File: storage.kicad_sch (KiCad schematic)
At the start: 26 parts, among them J4 uSD card, J5 uSD card, P1 uBUS2, P2 uBUS1, Q1 BC856, Q2 BC856, U10 IS61WV20488BLL-10TLI, U11 MT48LC16M16A2TG, U9 IS61WV20488BLL-10TLI

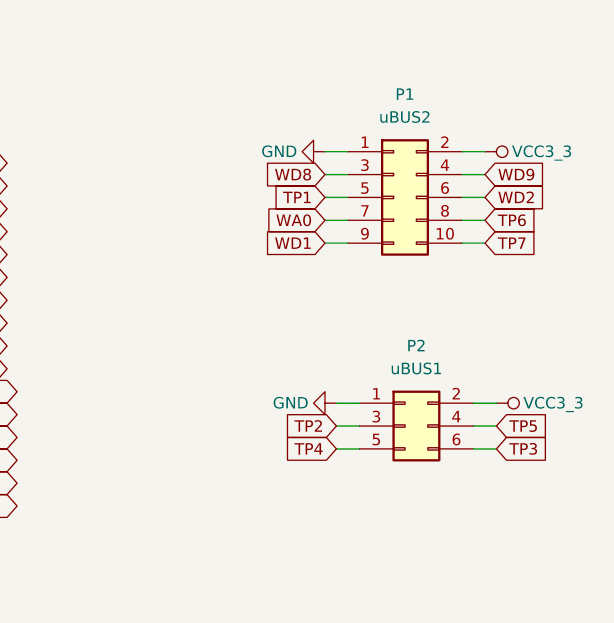
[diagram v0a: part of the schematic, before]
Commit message: Cleanup revA
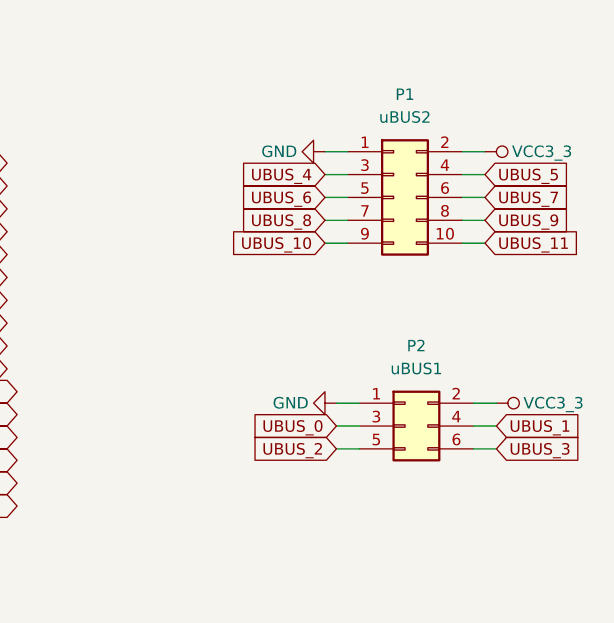
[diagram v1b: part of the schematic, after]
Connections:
- net TP1 renamed UBUS_6
- net TP2 renamed UBUS_0
- net TP3 renamed UBUS_3
- net TP4 renamed UBUS_2
- net TP5 renamed UBUS_1
- net TP6 renamed UBUS_9
- net TP7 renamed UBUS_11
- net WA0 renamed UBUS_8
- net WD1 renamed UBUS_10
- net WD2 renamed UBUS_7
- net WD8 renamed UBUS_4
- net WD9 renamed UBUS_5
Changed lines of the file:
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@@
     (effects (font (size 1.27 1.27)) (justify left bottom))
   )
-  (global_label "TP7" (shape input) (at 242.57 44.45 0) (fields_autoplaced)
-    (effects (font (size 1.27 1.27)) (justify left))
-    (property "Intersheetrefs" "${INTERSHEET_REFS}" (at 249.0023 44.45 0)
+  (global_label "UBUS_11" (shape input) (at 242.57 44.45 0) (fields_autoplaced)
+    (effects (font (size 1.27 1.27)) (justify left))
+    (property "Intersheetrefs" "${INTERSHEET_REFS}" (at 254.0823 44.45 0)
       (effects (font (size 1.27 1.27)) (justify left) hide)
     )
@@
     )
   )
-  (global_label "TP4" (shape input) (at 226.06 67.31 180) (fields_autoplaced)
-    (effects (font (size 1.27 1.27)) (justify right))
-    (property "Intersheetrefs" "${INTERSHEET_REFS}" (at 219.6277 67.31 0)
+  (global_label "UBUS_2" (shape input) (at 226.06 67.31 180) (fields_autoplaced)
+    (effects (font (size 1.27 1.27)) (justify right))
+    (property "Intersheetrefs" "${INTERSHEET_REFS}" (at 215.7572 67.31 0)
       (effects (font (size 1.27 1.27)) (justify right) hide)
     )
@@
     )
   )
-  (global_label "TP2" (shape input) (at 226.06 64.77 180) (fields_autoplaced)
-    (effects (font (size 1.27 1.27)) (justify right))
-    (property "Intersheetrefs" "${INTERSHEET_REFS}" (at 219.6277 64.77 0)
+  (global_label "UBUS_0" (shape input) (at 226.06 64.77 180) (fields_autoplaced)
+    (effects (font (size 1.27 1.27)) (justify right))
+    (property "Intersheetrefs" "${INTERSHEET_REFS}" (at 215.7572 64.77 0)
       (effects (font (size 1.27 1.27)) (justify right) hide)
     )
@@
     )
   )
-  (global_label "TP1" (shape input) (at 224.79 39.37 180) (fields_autoplaced)
-    (effects (font (size 1.27 1.27)) (justify right))
-    (property "Intersheetrefs" "${INTERSHEET_REFS}" (at 218.3577 39.37 0)
-      (effects (font (size 1.27 1.27)) (justify right) hide)
-    )
-  )
-  (global_label "TP6" (shape input) (at 242.57 41.91 0) (fields_autoplaced)
-    (effects (font (size 1.27 1.27)) (justify left))
-    (property "Intersheetrefs" "${INTERSHEET_REFS}" (at 249.0023 41.91 0)
+  (global_label "UBUS_6" (shape input) (at 224.79 39.37 180) (fields_autoplaced)
+    (effects (font (size 1.27 1.27)) (justify right))
+    (property "Intersheetrefs" "${INTERSHEET_REFS}" (at 214.4872 39.37 0)
+      (effects (font (size 1.27 1.27)) (justify right) hide)
+    )
+  )
+  (global_label "UBUS_9" (shape input) (at 242.57 41.91 0) (fields_autoplaced)
+    (effects (font (size 1.27 1.27)) (justify left))
+    (property "Intersheetrefs" "${INTERSHEET_REFS}" (at 252.8728 41.91 0)
       (effects (font (size 1.27 1.27)) (justify left) hide)
     )
@@
     )
   )
-  (global_label "WD8" (shape input) (at 224.79 36.83 180) (fields_autoplaced)
-    (effects (font (size 1.27 1.27)) (justify right))
-    (property "Intersheetrefs" "${INTERSHEET_REFS}" (at 217.8739 36.83 0)
+  (global_label "UBUS_4" (shape input) (at 224.79 36.83 180) (fields_autoplaced)
+    (effects (font (size 1.27 1.27)) (justify right))
+    (property "Intersheetrefs" "${INTERSHEET_REFS}" (at 214.4872 36.83 0)
       (effects (font (size 1.27 1.27)) (justify right) hide)
     )
@@
     )
   )
-  (global_label "WD9" (shape input) (at 242.57 36.83 0) (fields_autoplaced)
-    (effects (font (size 1.27 1.27)) (justify left))
-    (property "Intersheetrefs" "${INTERSHEET_REFS}" (at 249.4861 36.83 0)
+  (global_label "UBUS_5" (shape input) (at 242.57 36.83 0) (fields_autoplaced)
+    (effects (font (size 1.27 1.27)) (justify left))
+    (property "Intersheetrefs" "${INTERSHEET_REFS}" (at 252.8728 36.83 0)
       (effects (font (size 1.27 1.27)) (justify left) hide)
     )
@@
     )
   )
-  (global_label "WD1" (shape input) (at 224.79 44.45 180) (fields_autoplaced)
-    (effects (font (size 1.27 1.27)) (justify right))
-    (property "Intersheetrefs" "${INTERSHEET_REFS}" (at 217.8739 44.45 0)
+  (global_label "UBUS_10" (shape input) (at 224.79 44.45 180) (fields_autoplaced)
+    (effects (font (size 1.27 1.27)) (justify right))
+    (property "Intersheetrefs" "${INTERSHEET_REFS}" (at 213.2777 44.45 0)
       (effects (font (size 1.27 1.27)) (justify right) hide)
     )
@@
     )
   )
-  (global_label "WA0" (shape input) (at 224.79 41.91 180) (fields_autoplaced)
-    (effects (font (size 1.27 1.27)) (justify right))
-    (property "Intersheetrefs" "${INTERSHEET_REFS}" (at 218.0553 41.91 0)
+  (global_label "UBUS_8" (shape input) (at 224.79 41.91 180) (fields_autoplaced)
+    (effects (font (size 1.27 1.27)) (justify right))
+    (property "Intersheetrefs" "${INTERSHEET_REFS}" (at 214.4872 41.91 0)
       (effects (font (size 1.27 1.27)) (justify right) hide)
     )
@@
     )
   )
-  (global_label "TP5" (shape input) (at 243.84 64.77 0) (fields_autoplaced)
-    (effects (font (size 1.27 1.27)) (justify left))
-    (property "Intersheetrefs" "${INTERSHEET_REFS}" (at 250.2723 64.77 0)
+  (global_label "UBUS_1" (shape input) (at 243.84 64.77 0) (fields_autoplaced)
+    (effects (font (size 1.27 1.27)) (justify left))
+    (property "Intersheetrefs" "${INTERSHEET_REFS}" (at 254.1428 64.77 0)
       (effects (font (size 1.27 1.27)) (justify left) hide)
     )
@@
     )
   )
-  (global_label "WD2" (shape input) (at 242.57 39.37 0) (fields_autoplaced)
-    (effects (font (size 1.27 1.27)) (justify left))
-    (property "Intersheetrefs" "${INTERSHEET_REFS}" (at 249.4861 39.37 0)
+  (global_label "UBUS_7" (shape input) (at 242.57 39.37 0) (fields_autoplaced)
+    (effects (font (size 1.27 1.27)) (justify left))
+    (property "Intersheetrefs" "${INTERSHEET_REFS}" (at 252.8728 39.37 0)
       (effects (font (size 1.27 1.27)) (justify left) hide)
     )
@@
     )
   )
-  (global_label "TP3" (shape input) (at 243.84 67.31 0) (fields_autoplaced)
-    (effects (font (size 1.27 1.27)) (justify left))
-    (property "Intersheetrefs" "${INTERSHEET_REFS}" (at 250.2723 67.31 0)
-      (effects (font (size 1.27 1.27)) (justify left) hide)
-    )
+  (global_label "UBUS_3" (shape input) (at 243.84 67.31 0) (fields_autoplaced)
+    (effects (font (size 1.27 1.27)) (justify left))
+    (property "Intersheetrefs" "${INTERSHEET_REFS}" (at 254.1428 67.31 0)
+      (effects (font (size 1.27 1.27)) (justify left) hide)
+    )

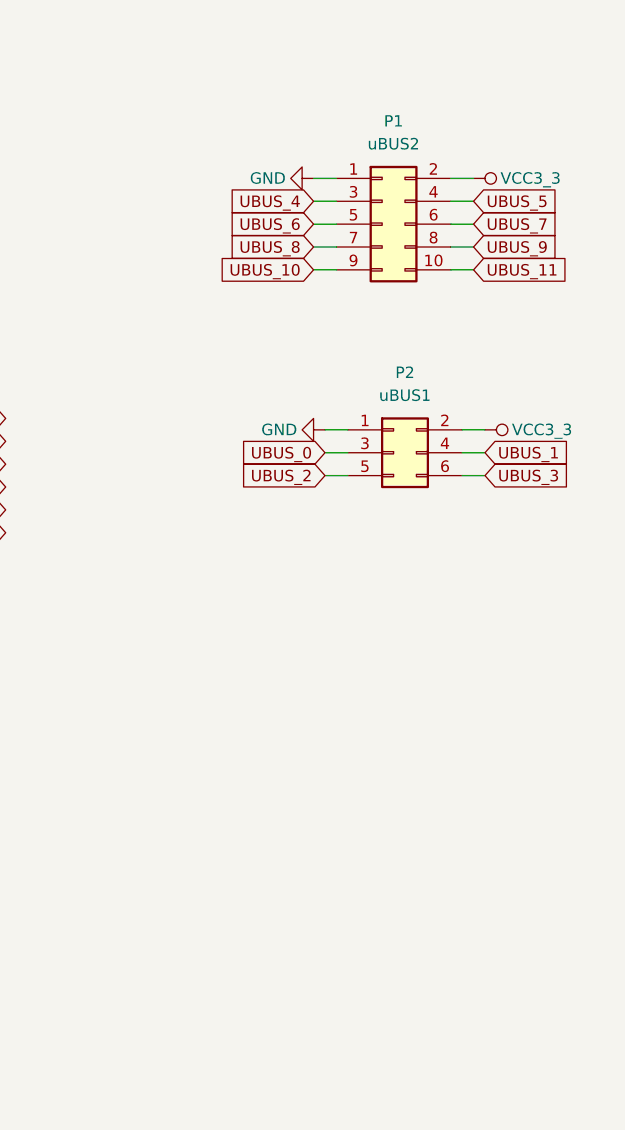
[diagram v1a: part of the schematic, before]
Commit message: Updated revB
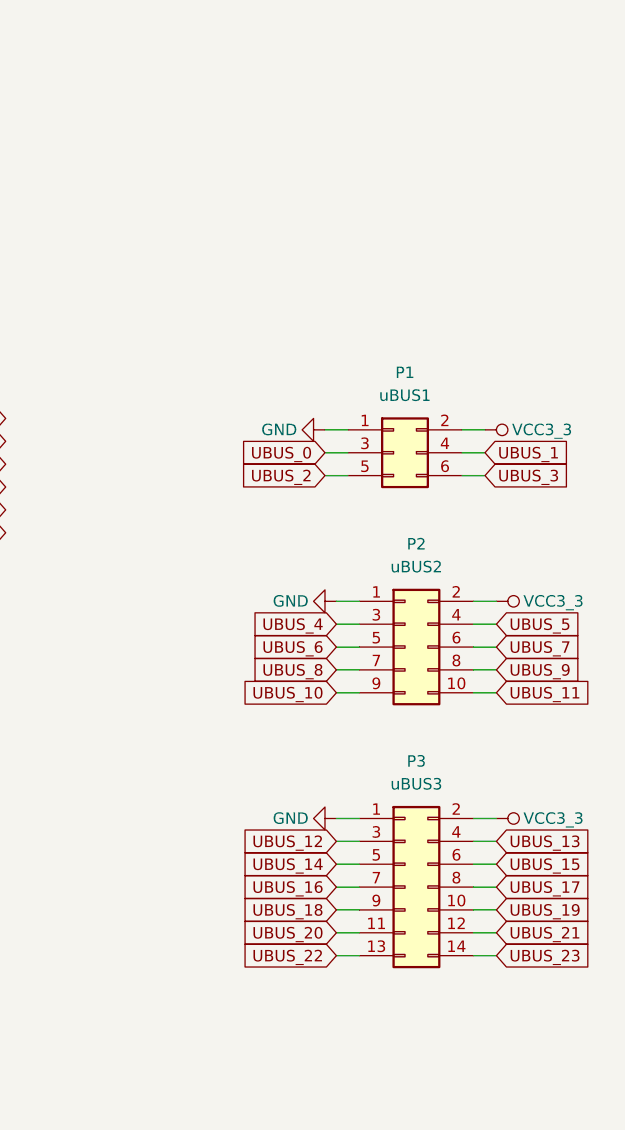
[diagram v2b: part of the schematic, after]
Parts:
- added P3: uBUS3, Connector_PinHeader_1.27mm:PinHeader_2x07_P1.27mm_Vertical, symbol Connector_Generic:Conn_02x07_Odd_Even
- renumbered P2 to P1, P1 to P2
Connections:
- net GND: now also P3.1 (Pin_1)
- net VCC3_3: now also P3.2 (Pin_2)
- new net UBUS_12: P3.3 (Pin_3)
- new net UBUS_13: P3.4 (Pin_4)
- new net UBUS_14: P3.5 (Pin_5)
- new net UBUS_15: P3.6 (Pin_6)
- new net UBUS_16: P3.7 (Pin_7)
- new net UBUS_17: P3.8 (Pin_8)
- new net UBUS_18: P3.9 (Pin_9)
- new net UBUS_19: P3.10 (Pin_10)
- new net UBUS_20: P3.11 (Pin_11)
- new net UBUS_21: P3.12 (Pin_12)
- new net UBUS_22: P3.13 (Pin_13)
- new net UBUS_23: P3.14 (Pin_14)
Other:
- moved on the sheet: P2
